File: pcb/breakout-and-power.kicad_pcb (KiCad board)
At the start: 2 copper layers, 45.8 x 55.7 mm, 61 parts, among them P1 CONN_01X02, P2 CONN_01X05, P3 CONN_01X10, P4 CONN_01X03, P5 CONN_01X12, P6 CONN_01X03, P7 CONN_01X03, P8 CONN_01X06, U1 TPS2420, U11 ADDI7013, U2 LT3487, U3 TPS63002, U7 TPS56x200, U8 LMZ10500

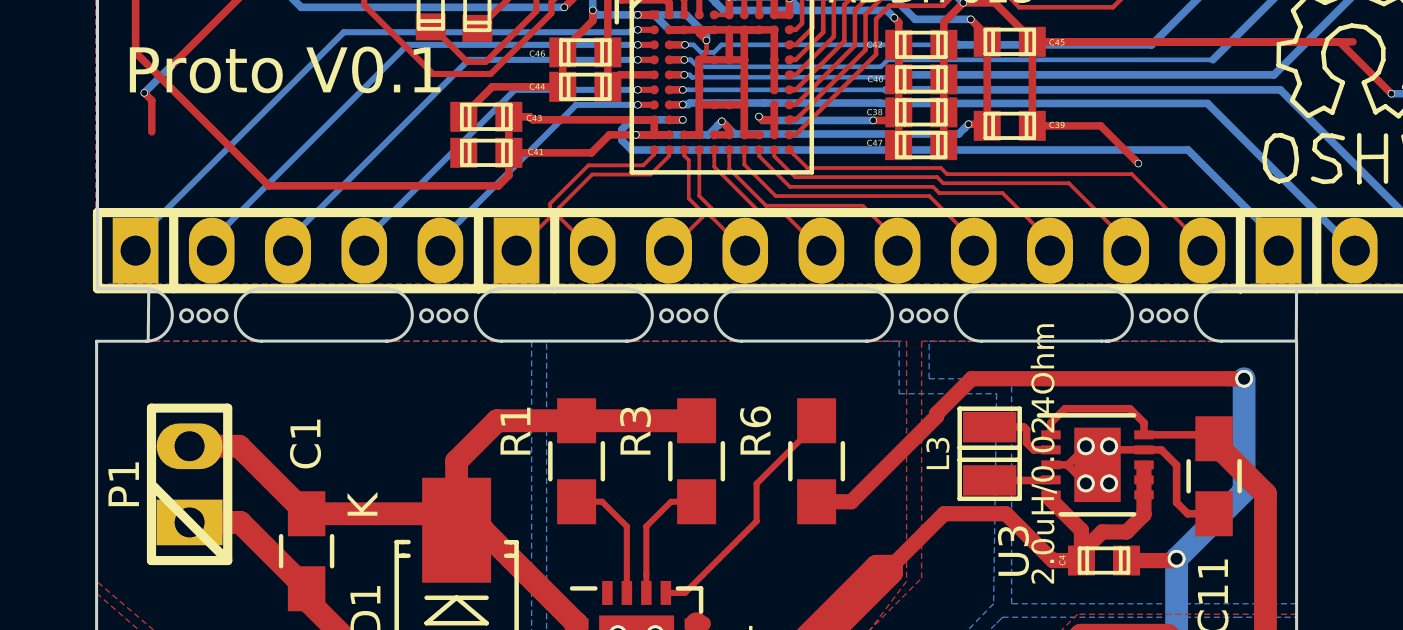
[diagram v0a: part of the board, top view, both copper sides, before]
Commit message: Start up work to revive this project.
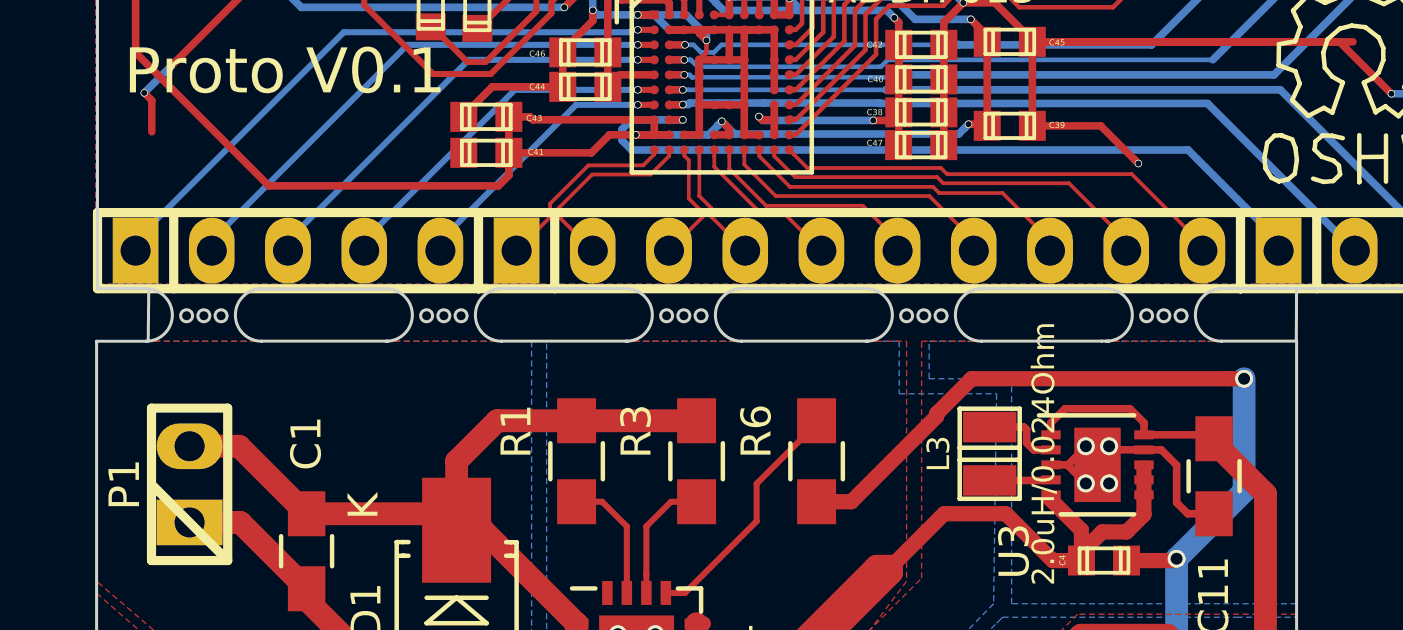
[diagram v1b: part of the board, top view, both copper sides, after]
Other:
- net class Default removed
